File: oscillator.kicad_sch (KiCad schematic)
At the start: 5 parts, among them Y1 ECS-2520MV-xxx-xx

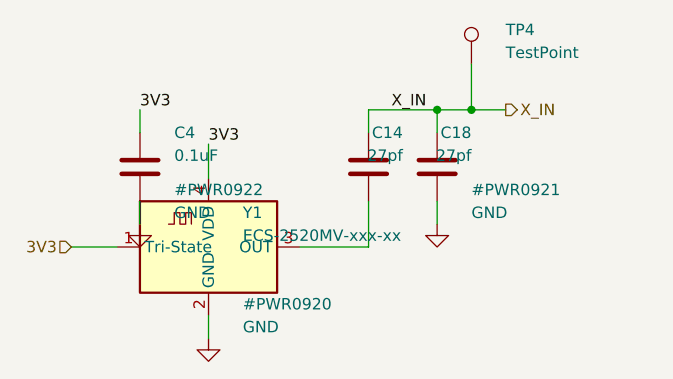
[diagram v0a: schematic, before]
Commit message: Migrate oscillator sheet to KL library symbols
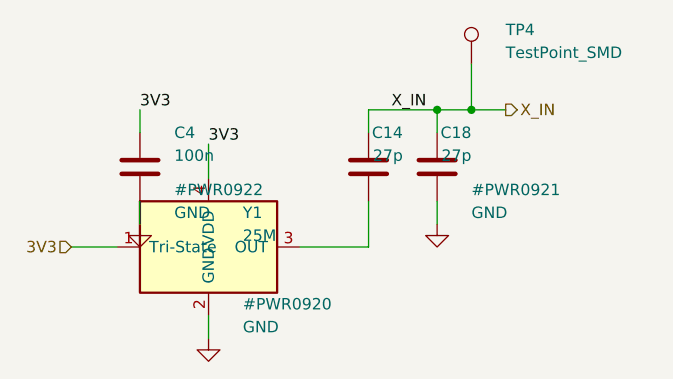
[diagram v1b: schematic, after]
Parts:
- C14, C18: value 27pf -> 27p; footprint Capacitor_SMD:C_0402_1005Metric_Pad0.74x0.62mm_HandSolder -> KL_Footprints:C_0402; symbol Device:C -> KL_C:C_27p_50V_5pct_C0G_0402; Dielectric (none) -> C0G; Digikey (none) -> TBD; LCSC (none) -> TBD; MPN (none) -> GRM1555C1H270JA01D; Mouser (none) -> 81-GRM1555C1H270JA01D; Package_in_inch (none) -> 0402; Tolerance_in_pct (none) -> 5; Voltage_in_V (none) -> 50
- C4: value 0.1uF -> 100n; footprint Capacitor_SMD:C_0402_1005Metric_Pad0.74x0.62mm_HandSolder -> KL_Footprints:C_0402; symbol Device:C -> KL_C:C_100n_35V_10pct_X7R_0402; Dielectric (none) -> X7R; Digikey (none) -> 445-6901-1-ND; LCSC (none) -> C2181802; MPN (none) -> CGA2B3X7R1V104K050BB; Mouser (none) -> 810-CGA2B3X7R1V104K; Package_in_inch (none) -> 0402; Tolerance_in_pct (none) -> 10; Voltage_in_V (none) -> 35
- TP4: value TestPoint -> TestPoint_SMD; footprint TestPoint:TestPoint_Pad_1.0x1.0mm -> KL_Footprints:TestPoint_SMD_1.0x1.0mm; symbol Connector:TestPoint -> KL_TestPoint:TestPoint_SMD
- Y1: value ECS-2520MV-xxx-xx -> 25M; footprint Oscillator:Oscillator_SMD_ECS_2520MV-xxx-xx-4Pin_2.5x2.0mm -> KL_Footprints:ECS-2520MV; symbol Oscillator:ECS-2520MV-xxx-xx -> KL_Oscillator:Oscillator_25M_25ppm_HCMOS_2.5x2.0; Digikey (none) -> TBD; Frequency_Stability_in_ppm (none) -> 25; LCSC (none) -> C405464; MPN (none) -> ECS-2520MV-250-CN-TR; Mouser (none) -> TBD; Output (none) -> HCMOS; Voltage_in_V (none) -> 1.6-3.6
